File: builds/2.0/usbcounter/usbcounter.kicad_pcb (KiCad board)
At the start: 2 copper layers, 91.4 x 61 mm, 49 parts, among them IC1 ATTINY826-XUR, J1 UJ2-MIBH-G-SMT-TR, J2 SMA, J3 Conn_Prog, J4 Conn_Disp, Q1 MMBT2222A, U1 FT230XS, U2 SN74LVC1Gxx, U3 MCP23008-xSO, U4 74LV8154, U5 NCP1117 3.3V, U6 MCP23008-xSO, Y1 14.7456 MHz TCXO

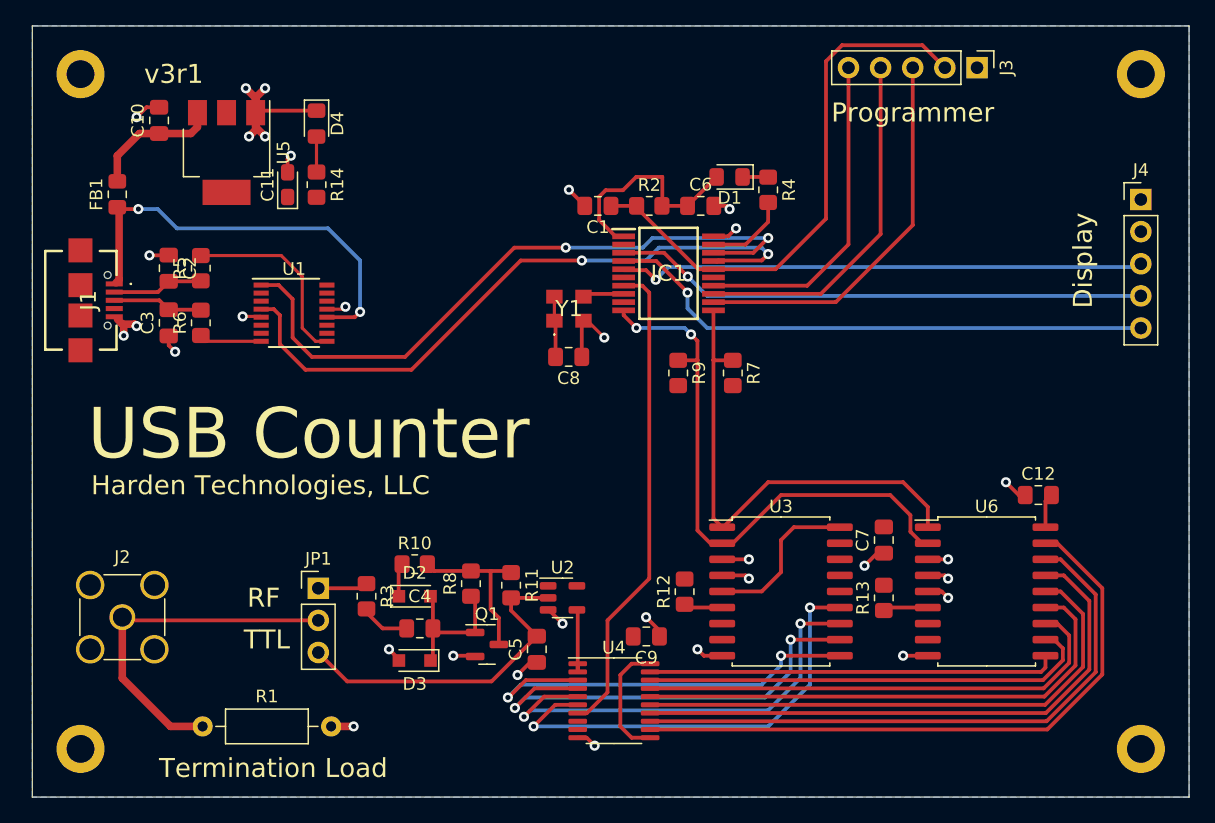
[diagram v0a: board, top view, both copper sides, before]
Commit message: 2.0: improve layout
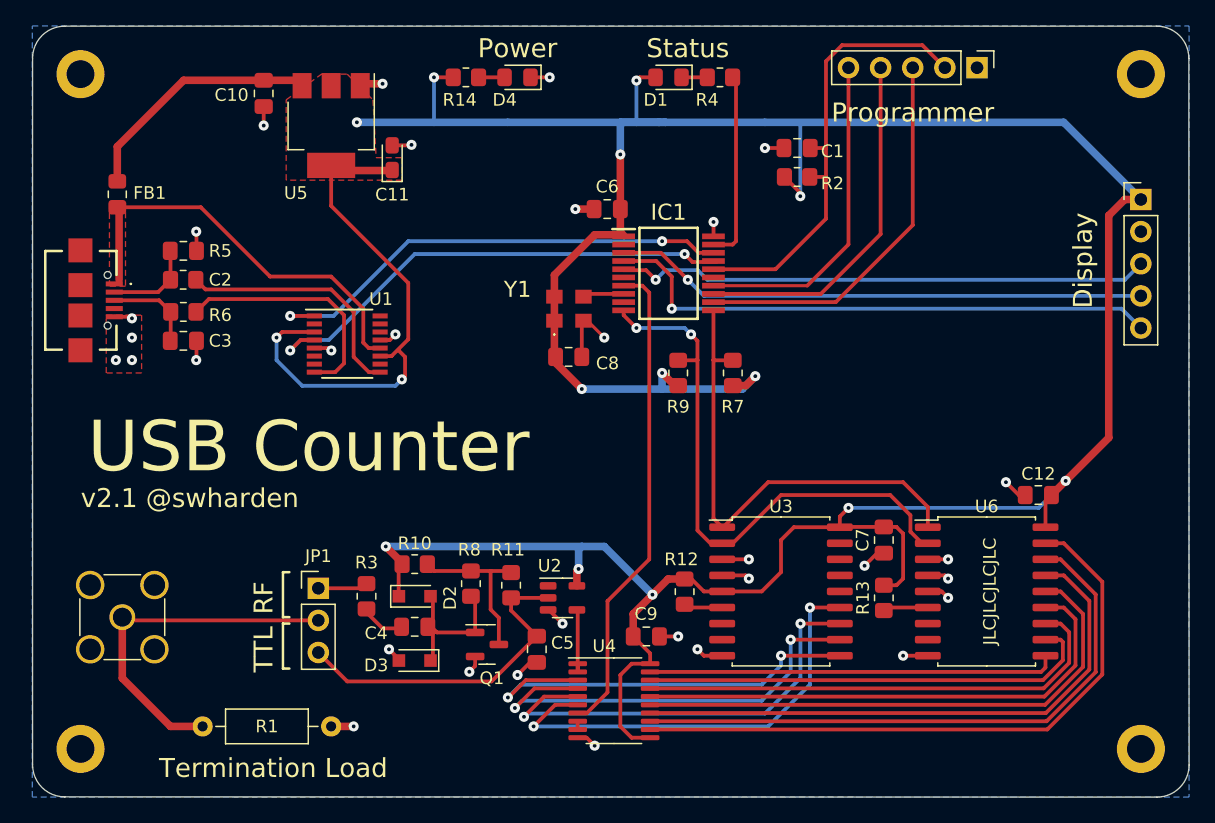
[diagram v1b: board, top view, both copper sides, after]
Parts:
- moved C1 16.4 mm to (111.3, 60.5)
- moved D4 16.3 mm to (89.2, 54.9), turned to 180 degrees
- moved R14 14.5 mm to (85.1, 54.9), turned to 180 degrees
- moved R2 11.9 mm to (111.3, 62.7), turned to 180 degrees
- moved R4 9.67 mm to (105.2, 54.9), turned to 0 degrees
- moved D1 9.24 mm to (101.1, 54.9)
- moved C11 8.54 mm to (79.2, 61.2)
- moved C10 8.54 mm to (69.1, 56.1), turned to -90 degrees
- moved U5 8.54 mm to (74.4, 58.7)
- moved C6 7.39 mm to (96.2, 65.3), turned to 180 degrees
- moved U1 4.86 mm to (75.7, 75.9)
- moved C3 1.83 mm to (62.7, 75.7), turned to 180 degrees
- moved C2 1.79 mm to (62.7, 68.6), turned to 180 degrees
- moved R5 1.67 mm to (62.7, 70.9), turned to 0 degrees
- moved R6 1.63 mm to (62.7, 73.4), turned to 180 degrees
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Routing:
- net VCC: track 50.3 -> 303.7 mm, vias 0 -> 15
- net PCTX: track 52.9 -> 38.2 mm
- net GND: track 65.5 -> 51.1 mm
- net Net-(R6-Pad1): track 4.96 -> 19.1 mm
- net PCRX: track 51.9 -> 39.4 mm
- net Net-(C10-Pad1): track 11.1 -> 19.7 mm
- net STATUS: track 6.61 -> 15.0 mm
- net RST: track 43.9 -> 36.2 mm
- net Net-(R5-Pad2): track 15.2 -> 19.7 mm
- net 5V: track 34.3 -> 32.7 mm, vias 2 -> 0
- net Net-(D4-Pad2): track 2.80 -> 2.06 mm
- net DISP_CLK: track 43.8 -> 44.6 mm
- net OVF: track 0.00 -> 0.65 mm
- net DISP_DAT: track 41.7 -> 42.4 mm
- net Net-(C5-Pad2): vias 1 -> 0
- added copper zone on F.Cu, net 5V
- added copper zone on F.Cu, net GND
- added copper zone on F.Cu, net VCC
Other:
- board size 91.4 x 61 mm -> 91.4 x 60.9 mm
- board text added: "JLCJLCJLCJLC"
- board text added: "Power"
- board text added: "Status"
- board text added: "v2.1 @swharden"
- board text removed: "Harden Technologies, LLC"
- board text removed: "v3r1"
